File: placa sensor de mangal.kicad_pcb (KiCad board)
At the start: 2 copper layers, 9.1 x 13.5 mm, 4 parts, among them J1 3, J2 1, J3 2

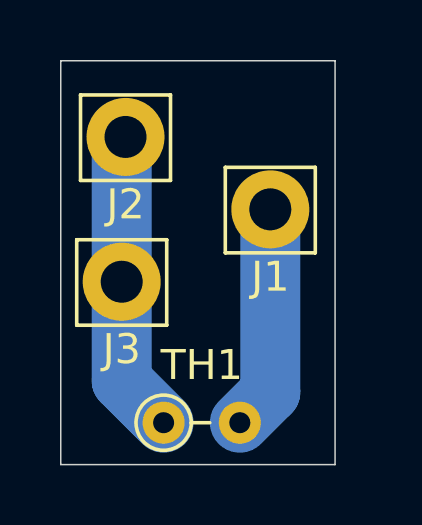
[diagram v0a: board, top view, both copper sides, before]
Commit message: sin cambios
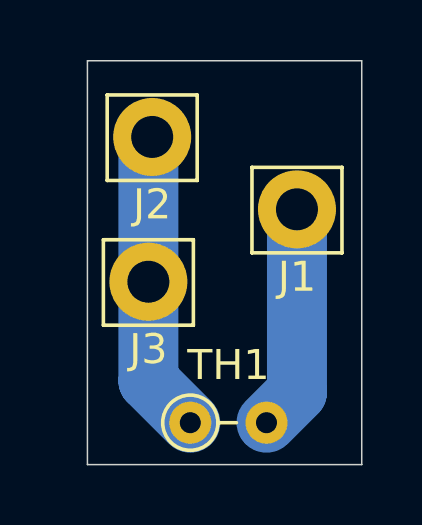
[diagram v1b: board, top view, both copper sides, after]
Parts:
- moved J1 0.89 mm to (146.1, 98.2)
- moved J3 0.89 mm to (141.1, 100.6)
- moved TH1 0.89 mm to (142.5, 105.3)
- moved J2 0.89 mm to (141.2, 95.8)
